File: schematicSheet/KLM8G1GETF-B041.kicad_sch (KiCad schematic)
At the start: 13 parts, among them U14 KLM8G1GETF-B041

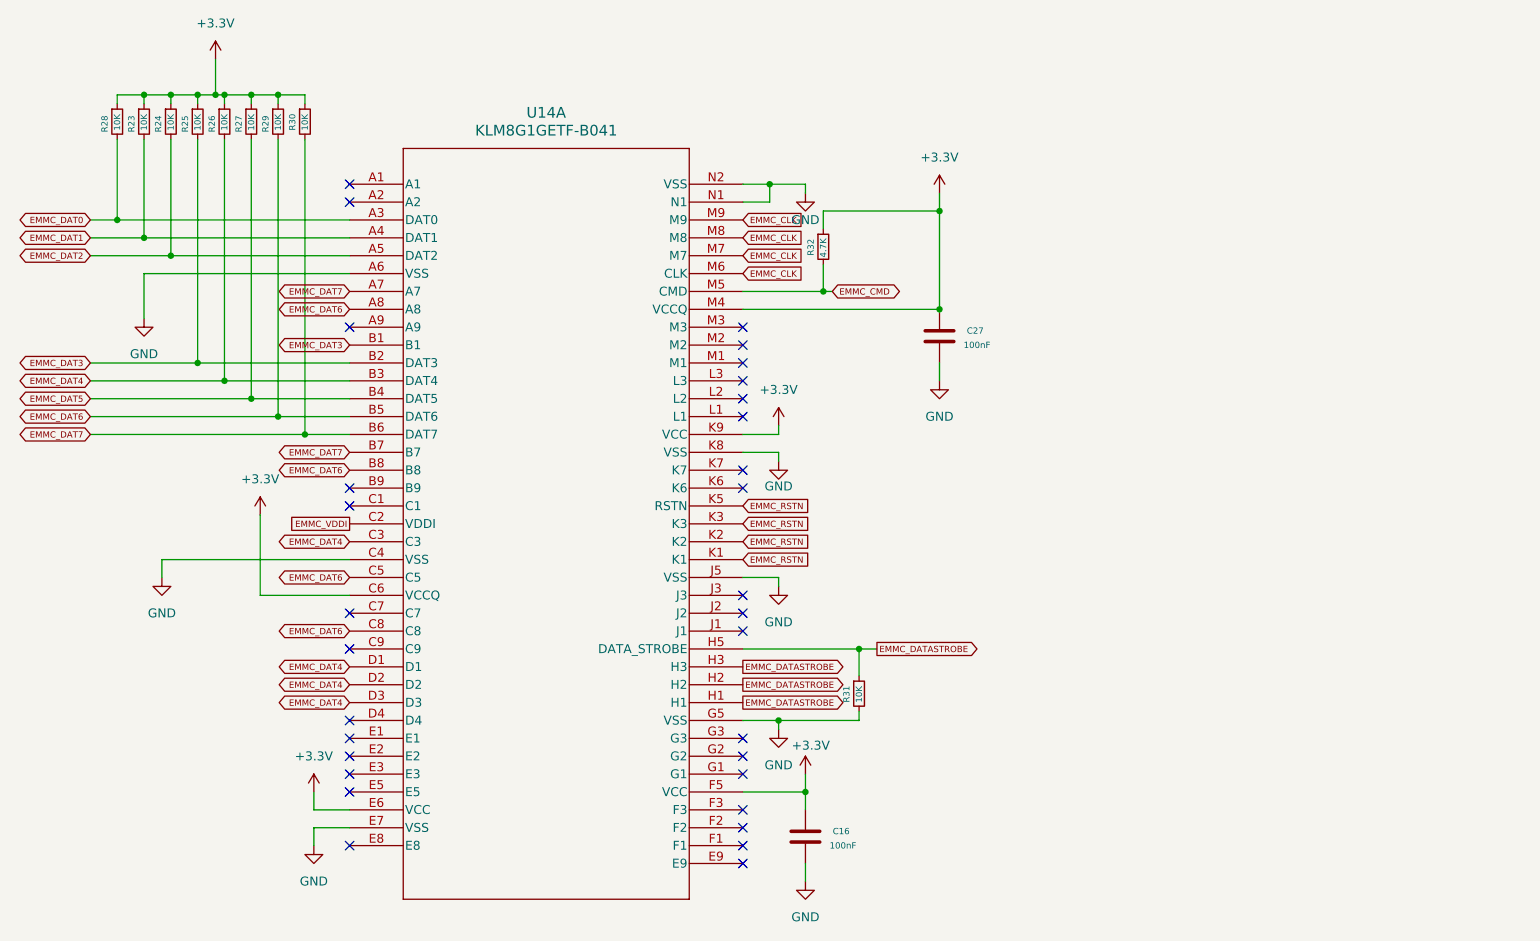
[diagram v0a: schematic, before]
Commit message: reroute
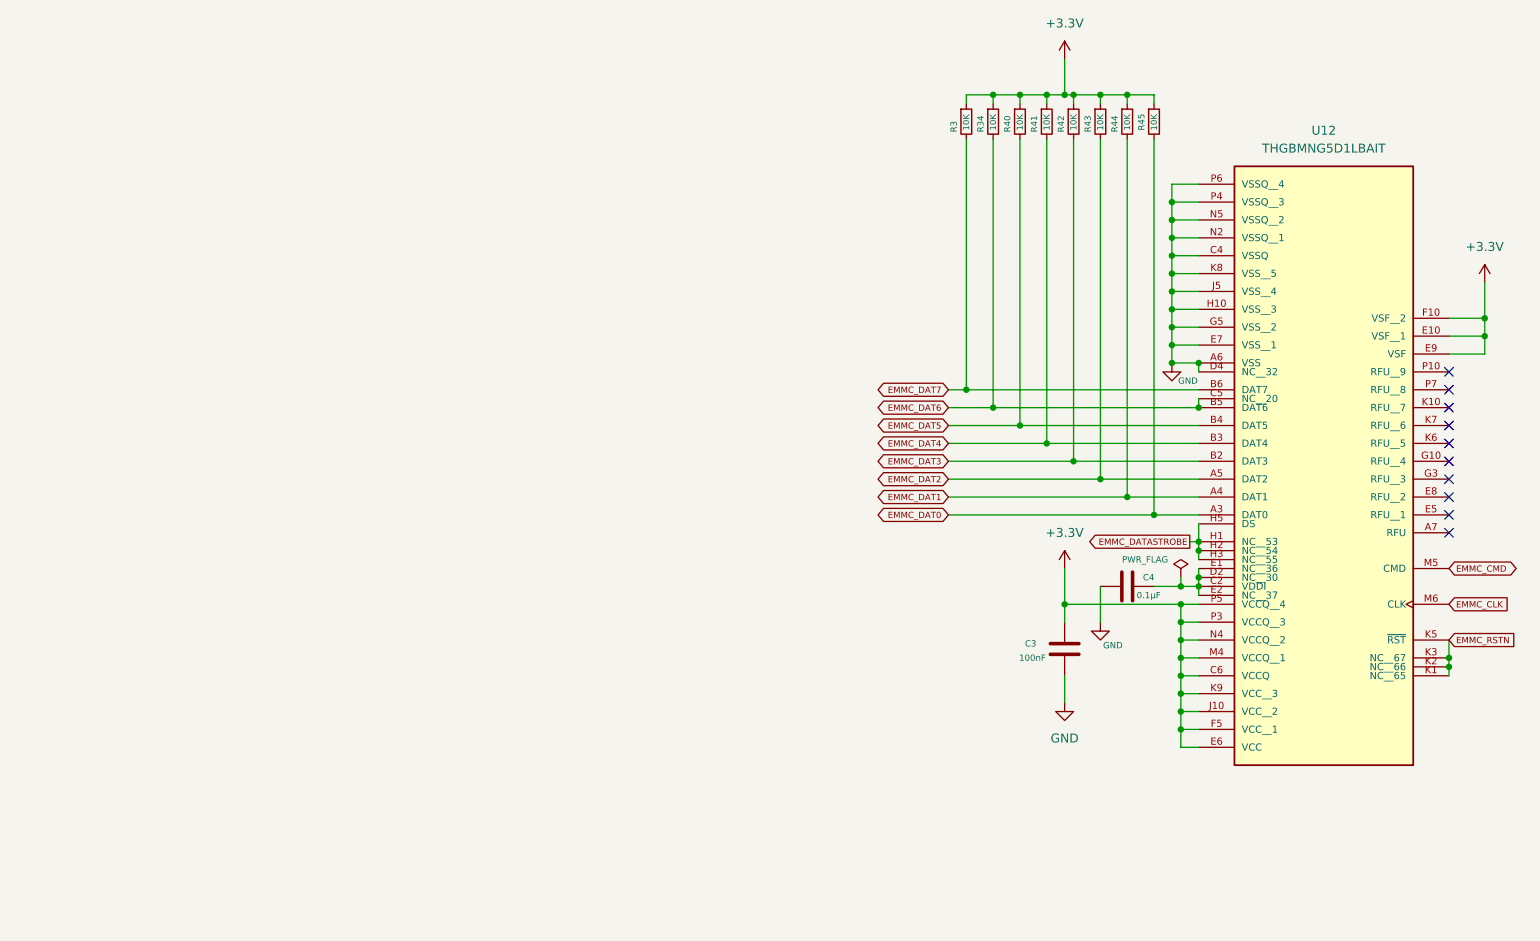
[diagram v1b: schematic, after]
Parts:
- removed C16, C27: 100nF, Capacitor_SMD:C_0402_1005Metric, symbol Device:C
- removed R23, R24, R25, R26, R27, R28, R29, R30, R31: 10K, Resistor_SMD:R_0402_1005Metric, symbol Device:R_Small
- removed R32: 4.7K, Resistor_SMD:R_0402_1005Metric, symbol Device:R_Small
- removed U14: KLM8G1GETF-B041, EMMC:KLMBG2JENB-B041_SAM, symbol EMMC:KLM8G1GETF-B041
- added C3: 100nF, Capacitor_SMD:C_0402_1005Metric, symbol Device:C
- added C4: 0.1µF, Capacitor_SMD:C_0402_1005Metric_Pad0.74x0.62mm_HandSolder, symbol Device:C
- added R3, R34, R40, R41, R42, R43, R44, R45: 10K, Resistor_SMD:R_0402_1005Metric, symbol Device:R_Small
- added U12: THGBMNG5D1LBAIT, EMMC:BGA153N50P14X14_1000X1100X80, symbol EMMC:THGBMNG5D1LBAIT
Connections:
- net +3.3V: now also C3.1, R3.1, R34.1, R40.1, R41.1, R42.1, R43.1, R44.1, R45.1, U12.C6 (VCCQ), U12.E10 (VSF__1), U12.E6 (VCC), U12.E9 (VSF), U12.F10 (VSF__2), U12.F5 (VCC__1), U12.J10 (VCC__2), U12.K9 (VCC__3), U12.M4 (VCCQ__1), U12.N4 (VCCQ__2), U12.P3 (VCCQ__3), U12.P5 (VCCQ__4)
- net EMMC_CLK: now also U12.M6 (CLK)
- net EMMC_CMD: now also U12.M5 (CMD)
- net EMMC_DAT0: now also R45.2, U12.A3 (DAT0)
- net EMMC_DAT1: now also R44.2, U12.A4 (DAT1)
- net EMMC_DAT2: now also R43.2, U12.A5 (DAT2)
- net EMMC_DAT3: now also R42.2, U12.B2 (DAT3)
- net EMMC_DAT4: now also R41.2, U12.B3 (DAT4)
- net EMMC_DAT5: now also R40.2, U12.B4 (DAT5)
- net EMMC_DAT6: now also R34.2, U12.B5 (DAT6), U12.C5 (NC__20)
- net EMMC_DAT7: now also R3.2, U12.B6 (DAT7)
- net EMMC_DATASTROBE: now also U12.H1 (NC__53), U12.H2 (NC__54), U12.H3 (NC__55), U12.H5 (DS)
- net EMMC_RSTN: now also U12.K1 (NC__65), U12.K2 (NC__66), U12.K3 (NC__67), U12.K5 (~{RST})
- net GND: now also C3.2, C4.1, U12.A6 (VSS), U12.C4 (VSSQ), U12.D4 (NC__32), U12.E7 (VSS__1), U12.G5 (VSS__2), U12.H10 (VSS__3), U12.J5 (VSS__4), U12.K8 (VSS__5), U12.N2 (VSSQ__1), U12.N5 (VSSQ__2), U12.P4 (VSSQ__3), U12.P6 (VSSQ__4)
- new net: C4.2, U12.C2 (VDDI), U12.D2 (NC__30), U12.E1 (NC__36), U12.E2 (NC__37)
- no-connect marks 31 -> 10
